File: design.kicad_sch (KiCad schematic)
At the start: 274 parts, among them J1 TYPE-C-31-M-12, U1 TTP223, U10 ATtiny1616-M, U2 TTP223, U3 TTP223, U4 TTP223, U5 TTP223, U6 TTP223, U7 TTP223, U8 TTP223, U9 MAX77751CEFG_T

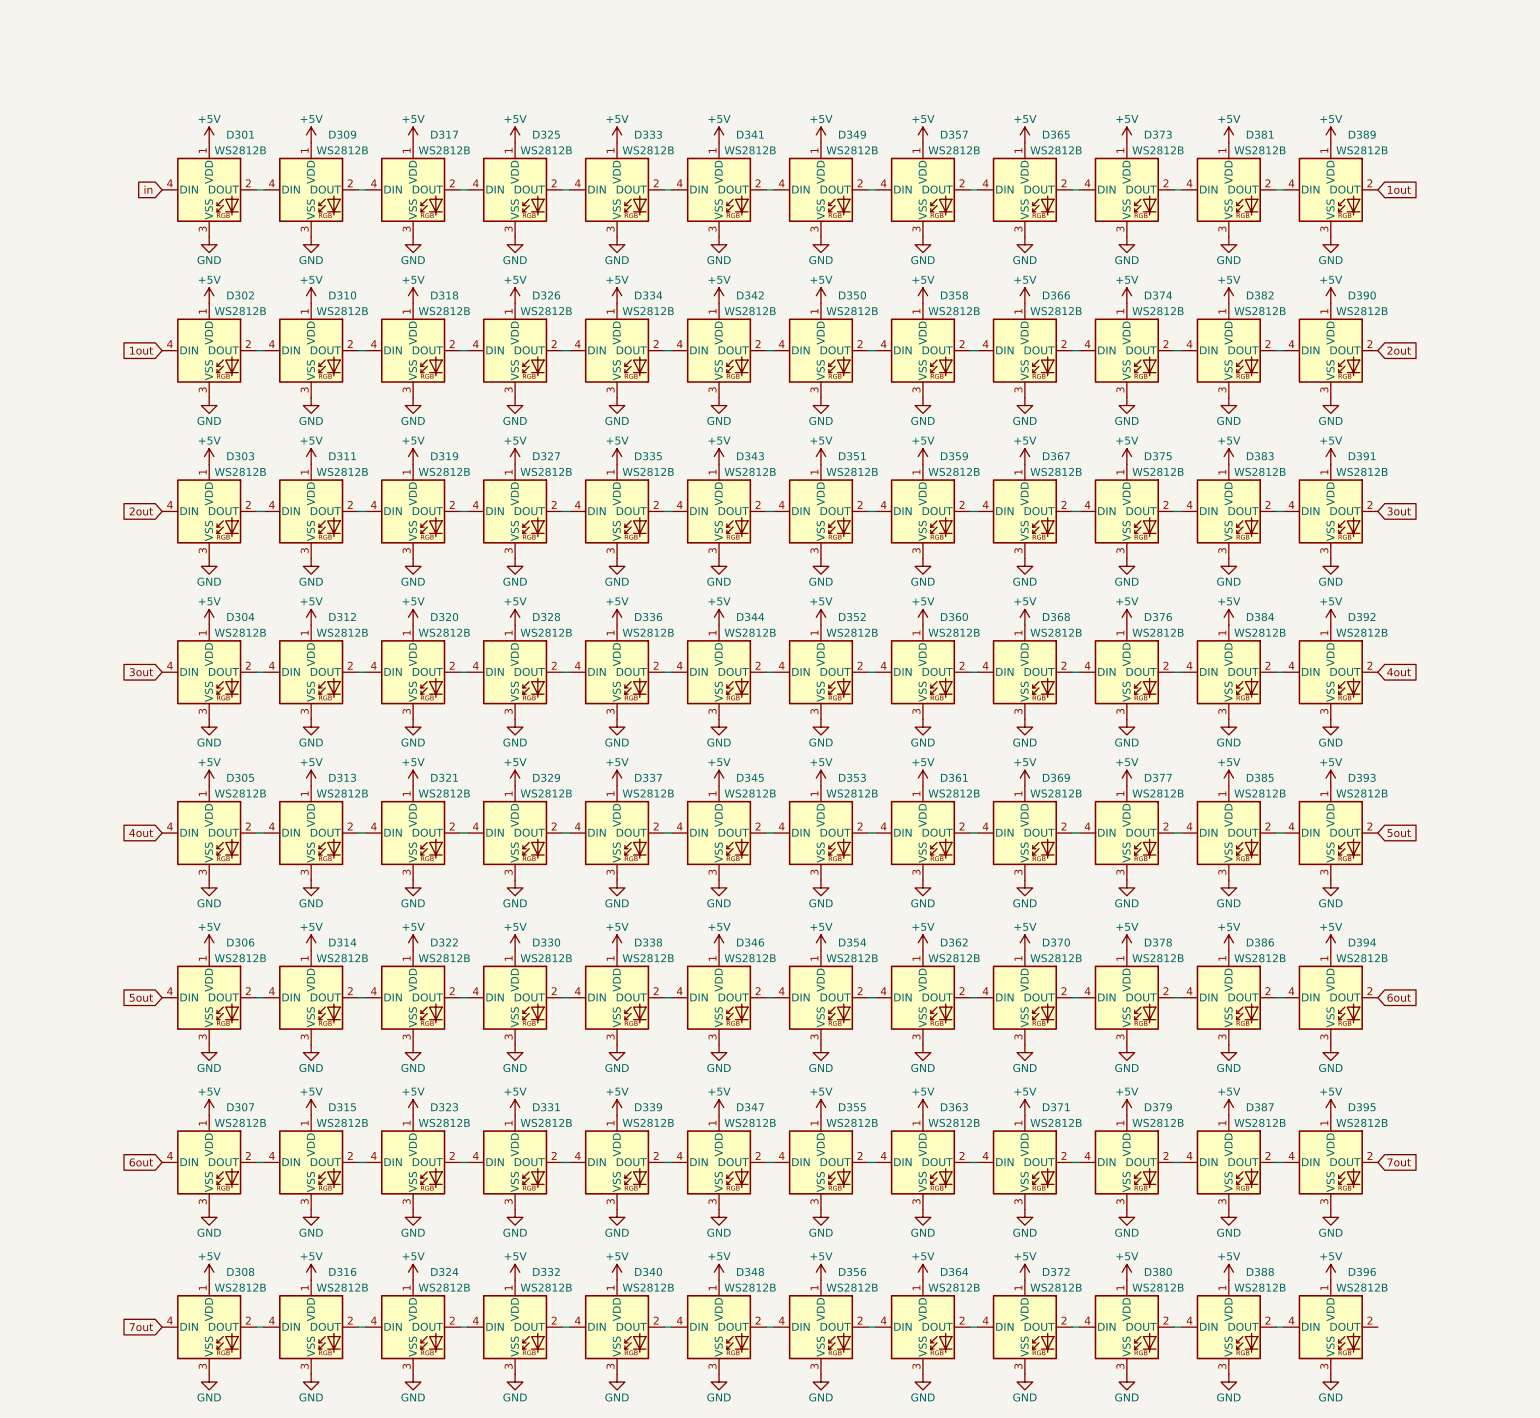
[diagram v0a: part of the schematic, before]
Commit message: new layout
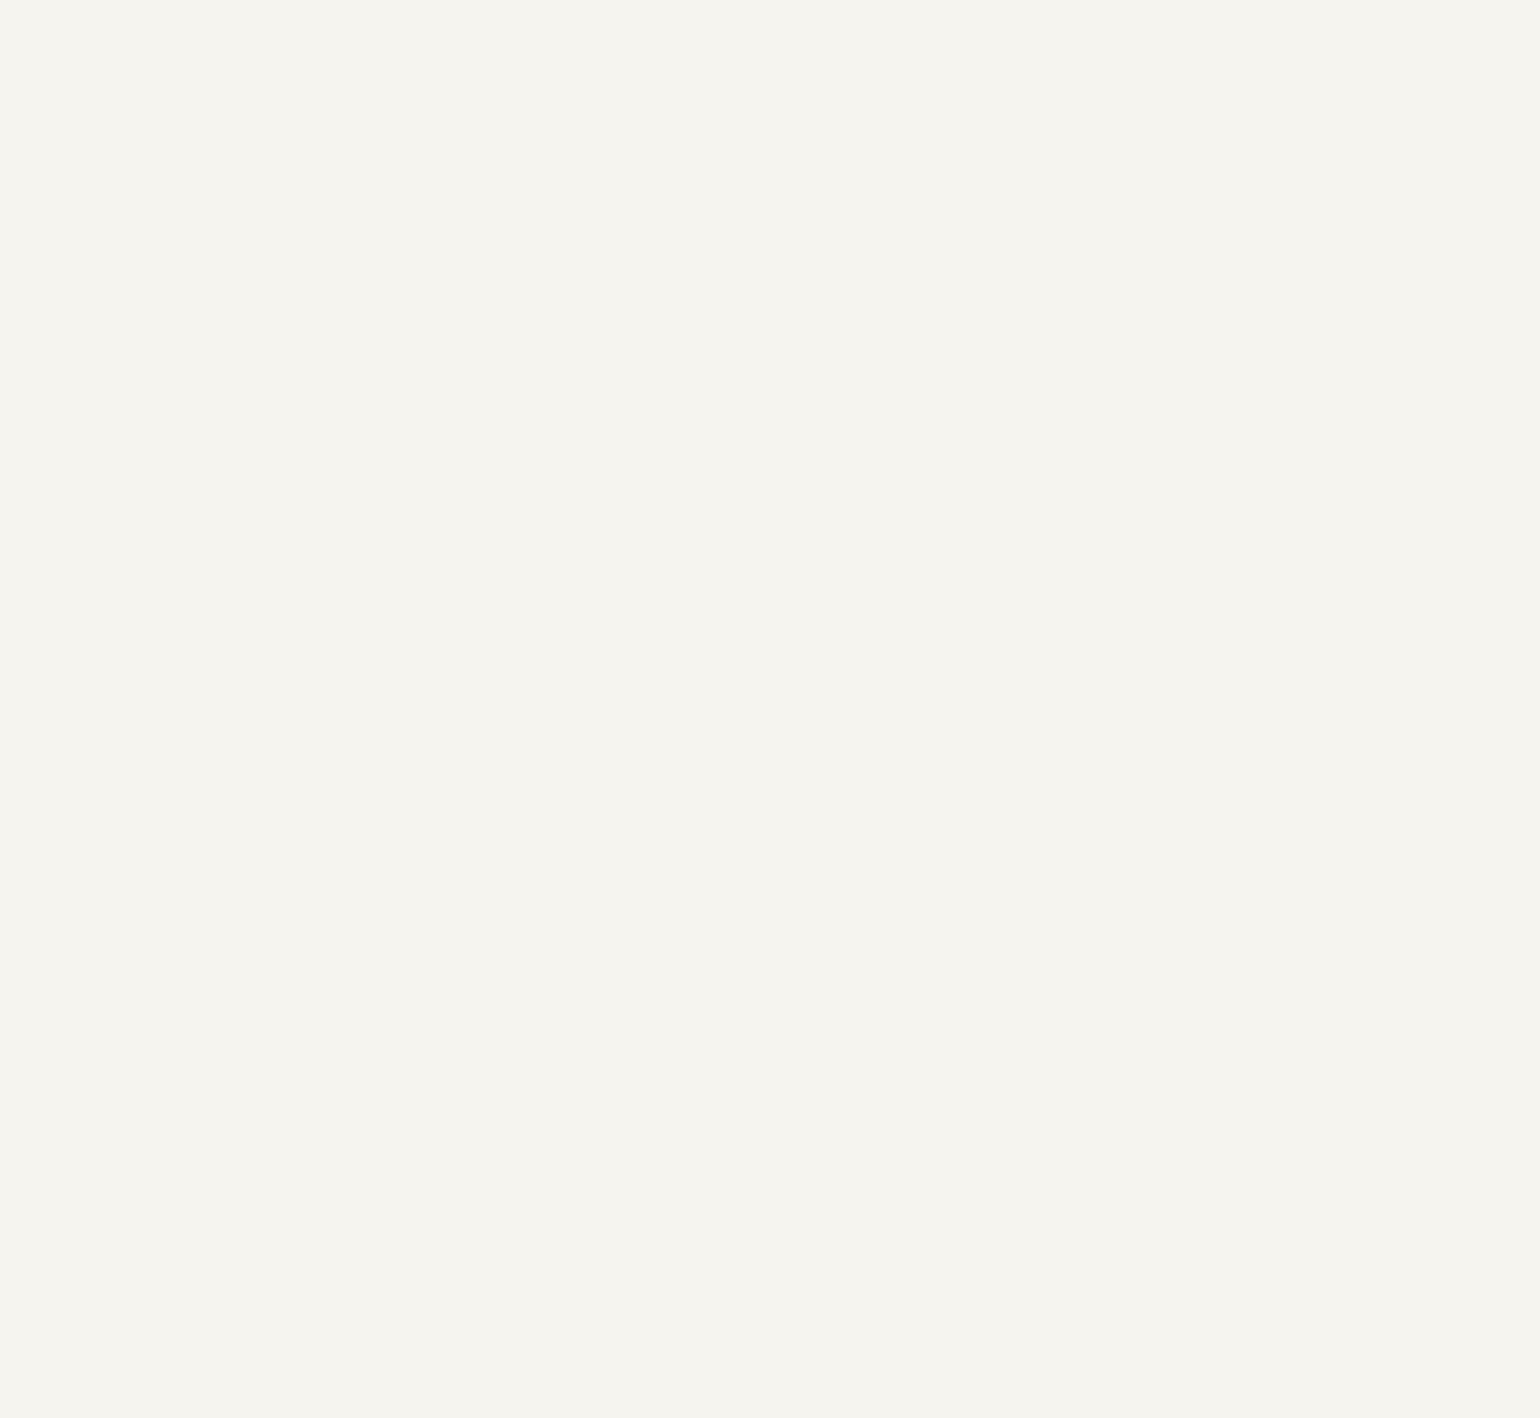
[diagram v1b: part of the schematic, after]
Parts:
- removed D301, D302, D303, D304, D305, D306, D307, D308, D309, D310, D311, D312, D313, D314, D315, D316, D317, D318, D319, D320, D321, D322, D323, D324, D325, D326, D327, D328, D329, D330, D331, D332, D333, D334, D335, D336, D337, D338, D339, D340, D341, D342, D343, D344, D345, D346, D347, D348, D349, D350, D351, D352, D353, D354, D355, D356, D357, D358, D359, D360, D361, D362, D363, D364, D365, D366, D367, D368, D369, D370, D371, D372, D373, D374, D375, D376, D377, D378, D379, D380, D381, D382, D383, D384, D385, D386, D387, D388, D389, D390, D391, D392, D393, D394, D395, D396: WS2812B, LED_SMD:LED_WS2812B_PLCC4_5.0x5.0mm_P3.2mm, symbol LED:WS2812B

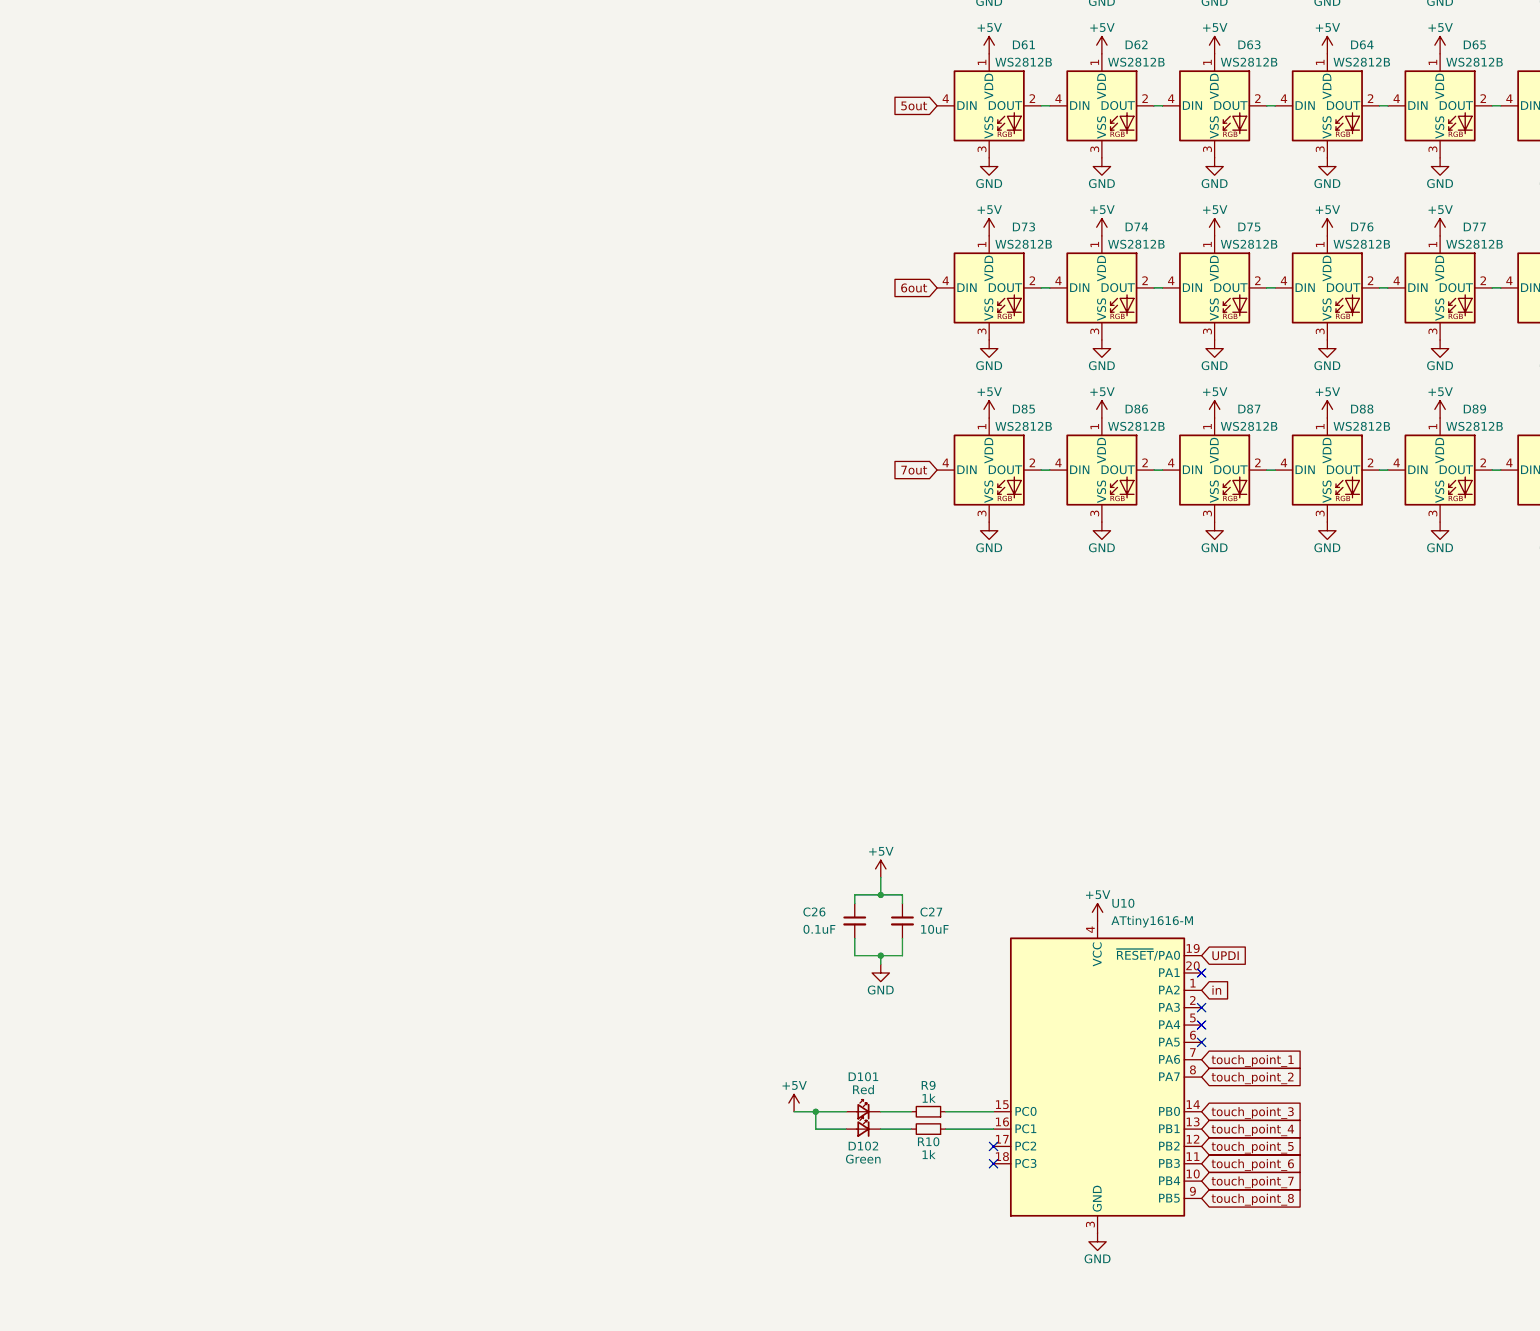
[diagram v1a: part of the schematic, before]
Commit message: updates
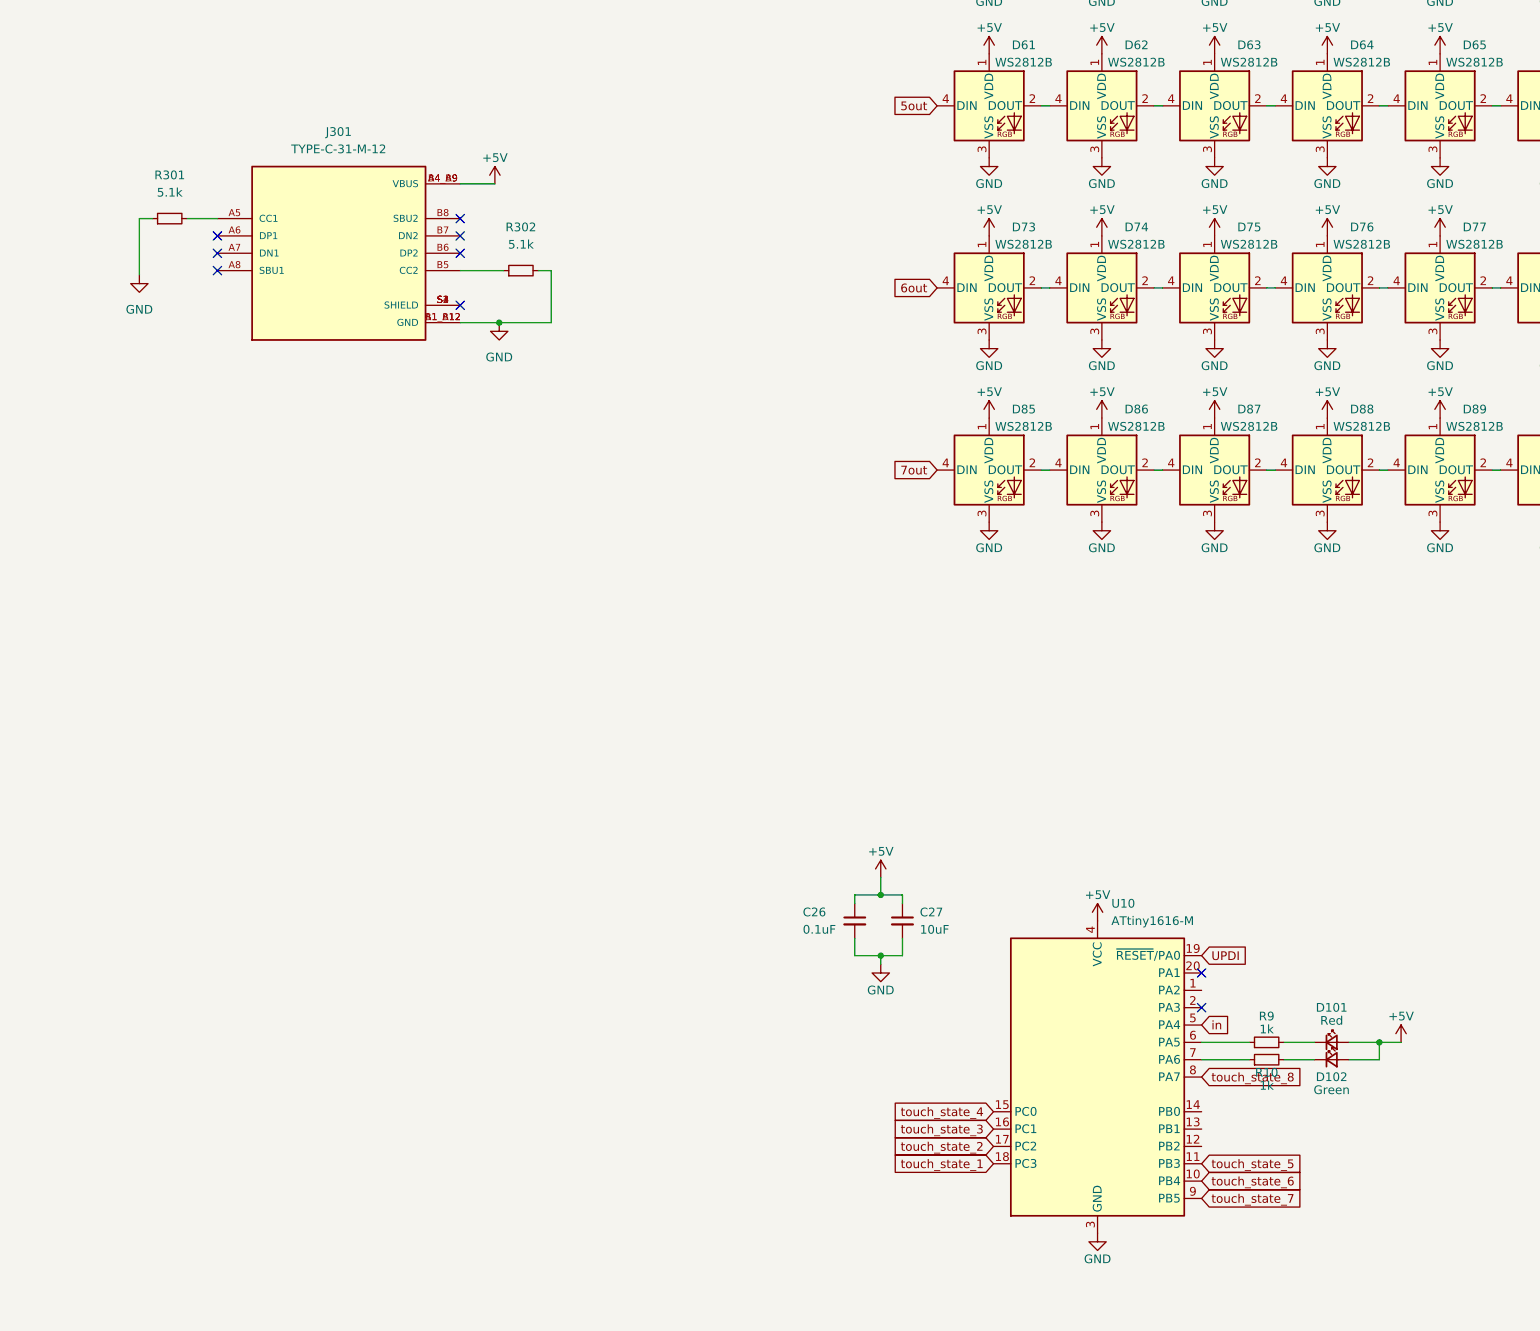
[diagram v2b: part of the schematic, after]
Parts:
- added J301: TYPE-C-31-M-12, Snapeda:TYPE-C-31-M-12_HRO_TYPE-C-31-M-12, symbol Snapeda:TYPE-C-31-M-12
- added R301, R302: 5.1k, Resistor_SMD:R_0805_2012Metric, symbol Device:R_Small
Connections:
- net +5V: now also J301.A4_B9 (VBUS), J301.B4_A9 (VBUS)
- net GND: now also J301.A1_B12 (GND), J301.B1_A12 (GND), R301.1, R302.2
- net in: now also U10.5 (PA4); no longer U10.1 (PA2)
- net touch_point_1: no longer U10.7 (PA6)
- net touch_point_2: no longer U10.8 (PA7)
- net touch_point_3: no longer U10.14 (PB0)
- net touch_point_4: no longer U10.13 (PB1)
- net touch_point_5: no longer U10.12 (PB2)
- net touch_point_6: no longer U10.11 (PB3)
- net touch_point_7: no longer U10.10 (PB4)
- net touch_point_8: no longer U10.9 (PB5)
- net touch_state_1: now also U10.18 (PC3)
- net touch_state_2: now also U10.17 (PC2)
- net touch_state_3: now also U10.16 (PC1)
- net touch_state_4: now also U10.15 (PC0)
- net touch_state_5: now also U10.11 (PB3)
- net touch_state_6: now also U10.10 (PB4)
- net touch_state_7: now also U10.9 (PB5)
- net touch_state_8: now also U10.8 (PA7)
- net at R9.1: now also U10.6 (PA5); no longer U10.15 (PC0)
- net at R10.1: now also U10.7 (PA6); no longer U10.16 (PC1)
- new net: J301.A5 (CC1), R301.2
- new net: J301.B5 (CC2), R302.1
- new net: J301.S1 (SHIELD), J301.S2 (SHIELD), J301.S3 (SHIELD), J301.S4 (SHIELD)
- no-connect marks 9 -> 12
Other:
- moved on the sheet: D101, D102, R10, R9
